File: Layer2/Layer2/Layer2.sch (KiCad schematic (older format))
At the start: 34 parts, among them J1 Conn_02x20_Odd_Even, J2 Conn_02x20_Odd_Even, U1 74LS08, U10 74HC245, U11 74HC245, U12 74LS181, U13 28C256, U14 74LS173, U15 628128_DIP32_SSOP32, U16 74LS173, U17 74LS85, U18 74LS08, U19 74LS273, U2 74HC273, U20 74LS273, U3 74HC273, U4 74HC273, U5 74HC245, U6 74HC245, U7 74HC245, U8 74LS181, U9 74HC273

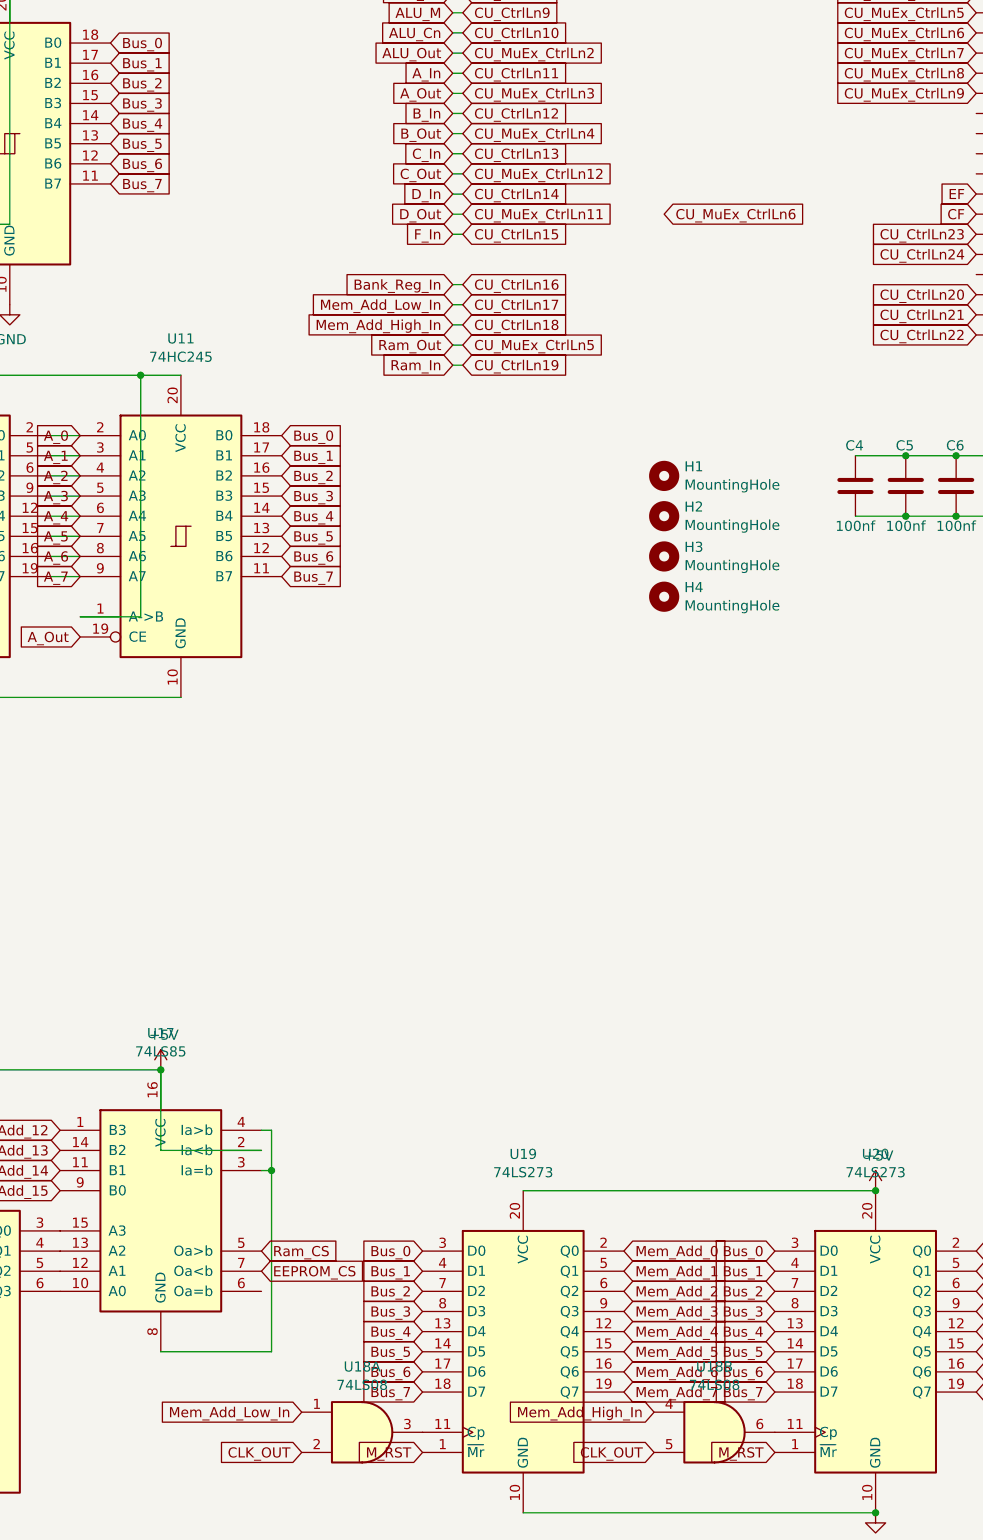
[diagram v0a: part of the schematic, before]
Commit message: Layer 3 complete
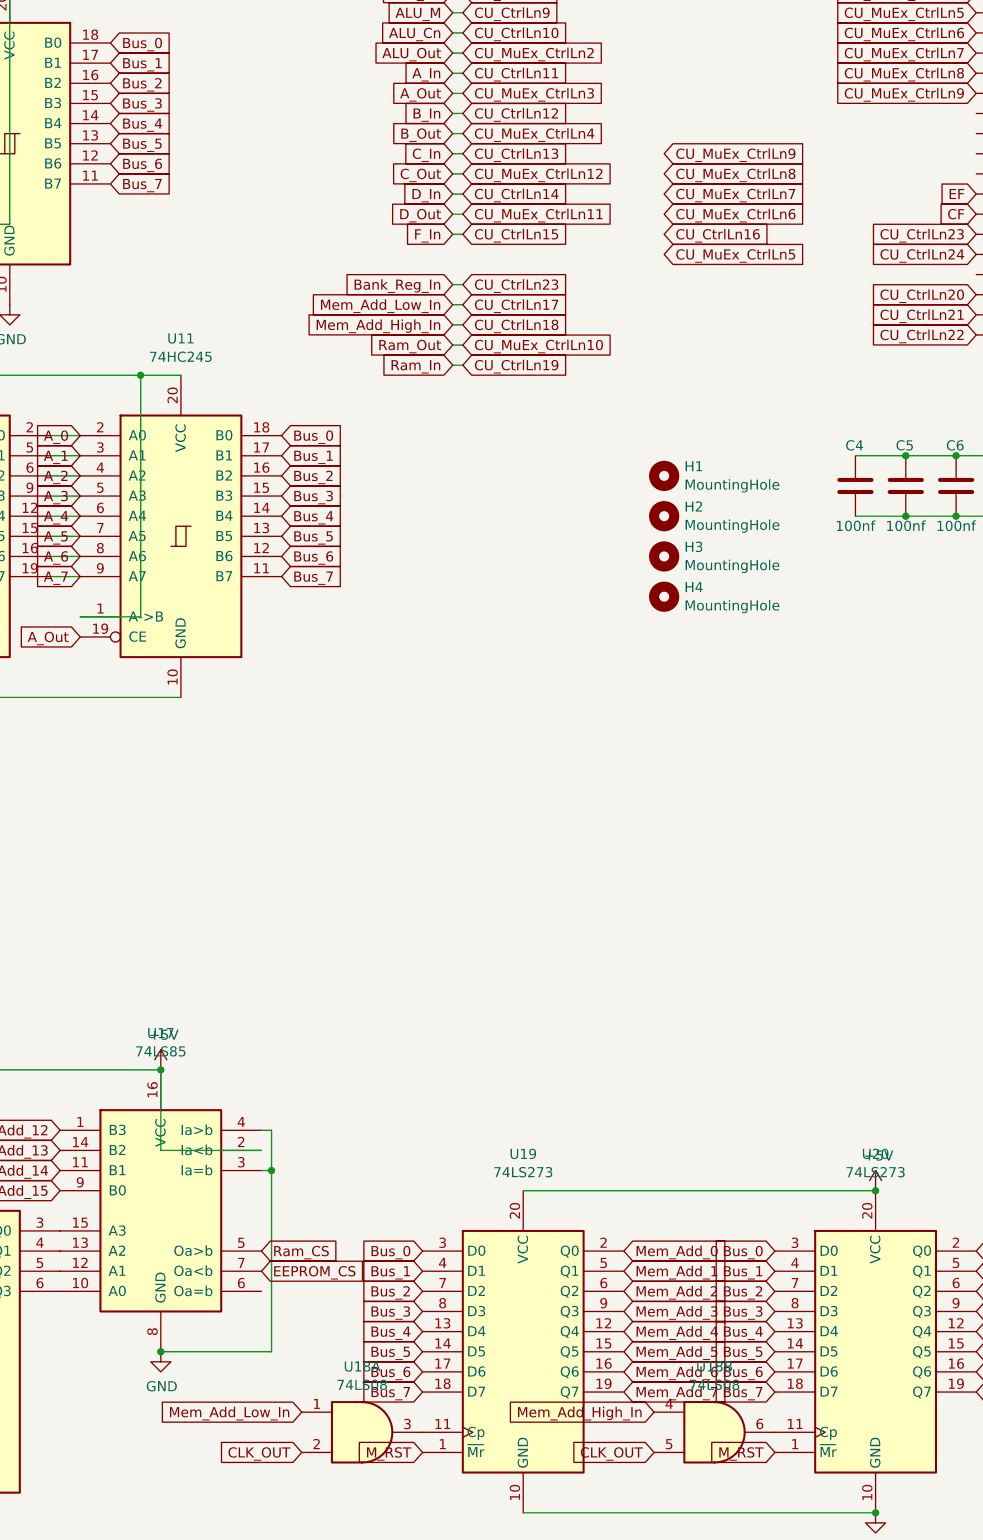
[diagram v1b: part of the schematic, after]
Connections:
- net CU_CtrlLn23 is gone; now on net Bank_Reg_In: J2.29 (Pin_29)
- net Bank_Reg_In: no longer J1.24 (Pin_24)
- net CU_MuEx_CtrlLn10: now also U13.22 (~OE), U15.24 (~OE)
- net CU_MuEx_CtrlLn5: no longer U13.22 (~OE), U15.24 (~OE)
- net GND: now also U17.3 (Ia=b), U17.4 (Ia>b), U17.8 (GND)
- new net CU_CtrlLn16: J1.24 (Pin_24)
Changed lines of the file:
@@
 EESchema Schematic File Version 4
+LIBS:Layer2-cache
 EELAYER 30 0
 EELAYER END
@@
 Text GLabel 7300 4100 2    50   Input ~ 0
 CU_MuEx_CtrlLn4
-Text GLabel 7300 5150 2    50   Input ~ 0
+Text GLabel 8300 4700 2    50   Input ~ 0
 CU_MuEx_CtrlLn5
 Text GLabel 8300 4500 2    50   Input ~ 0
@@
 Text GLabel 7250 5150 0    50   Input ~ 0
 Ram_Out
-Text GLabel 7300 4850 2    50   Input ~ 0
+Text GLabel 8300 4600 2    50   Input ~ 0
 CU_CtrlLn16
 Text GLabel 7300 5050 2    50   Input ~ 0
@@
 Wire Wire Line
 	7250 5250 7300 5250
+Text GLabel 7300 4850 2    50   Input ~ 0
+CU_CtrlLn23
+Text GLabel 7300 5150 2    50   Input ~ 0
+CU_MuEx_CtrlLn10
+$Comp
+L power:GND #PWR?
+U 1 1 626DBD5B
+P 5800 10150
+F 0 "#PWR?" H 5800 9900 50  0001 C CNN
+F 1 "GND" H 5805 9977 50  0000 C CNN
+F 2 "" H 5800 10150 50  0001 C CNN
+F 3 "" H 5800 10150 50  0001 C CNN
+	1    5800 10150
+	1    0    0    -1
+$EndComp
+Connection ~ 5800 10150
+Text GLabel 8300 4400 2    50   Input ~ 0
+CU_MuEx_CtrlLn7
+Text GLabel 8300 4300 2    50   Input ~ 0
+CU_MuEx_CtrlLn8
+Text GLabel 8300 4200 2    50   Input ~ 0
+CU_MuEx_CtrlLn9
 $EndSCHEMATC

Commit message: Backup
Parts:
- removed U18: 74LS08, Package_DIP:DIP-14_W7.62mm_LongPads, symbol 74xx:74LS08
- added U?: 74f543, symbol Connector_Generic:Conn_02x12_Counter_Clockwise
- added U? (x5): 7400, symbol 74xx:7400
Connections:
- net labels added: KF
- wire segments 129 -> 145
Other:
- moved on the sheet: U16, U17, U19, U1B, U1C, U1E, U20, U3, U4, U6, U7
